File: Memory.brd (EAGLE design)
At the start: 106.7 x 54.3 mm, 14 parts, among them IC1 AT28C256ZIF, IC2 HM62256DIP, IC3 74LS139N, IC4 HM62256DIP

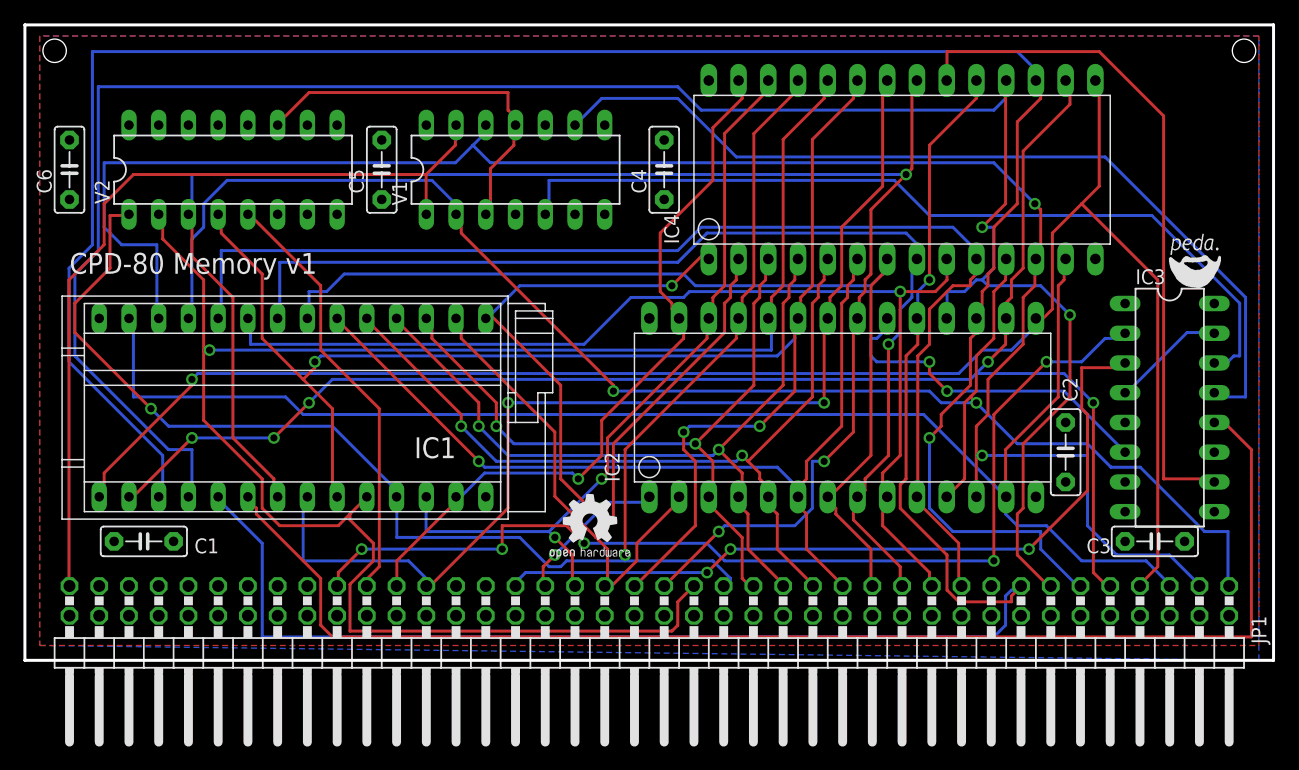
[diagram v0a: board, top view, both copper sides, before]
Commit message: Update Memory
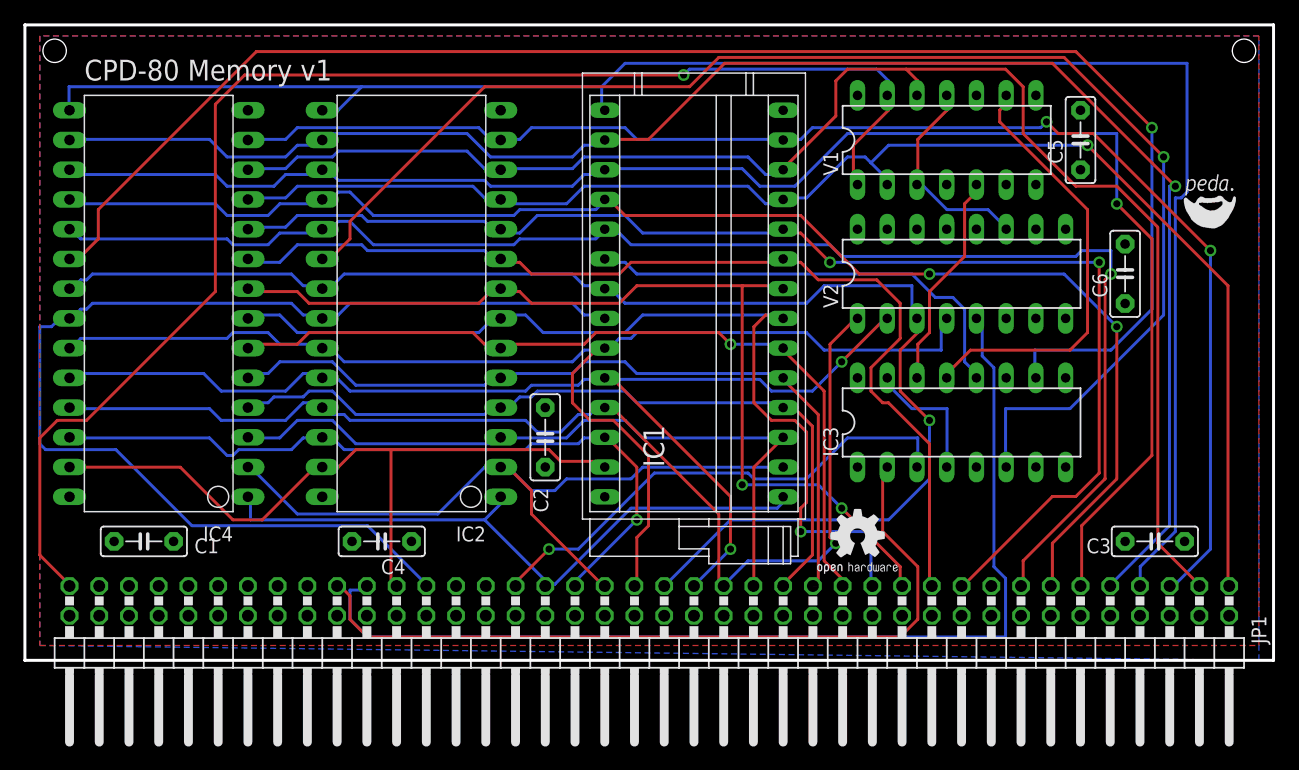
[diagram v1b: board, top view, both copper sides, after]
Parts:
- moved C6 90.6 mm to (92.7, 33.0)
- moved V2 62.9 mm to (78.7, 33.0)
- moved C5 59.7 mm to (88.9, 44.5)
- moved IC4 52.7 mm to (15.2, 22.9), turned to 90 degrees
- moved C2 44.5 mm to (43.2, 19.1), turned to 270 degrees
- moved C4 39.9 mm to (29.2, 10.2), turned to 180 degrees
- moved V1 36.9 mm to (77.5, 44.5)
- moved IC1 35.4 mm to (55.9, 30.5), turned to 90 degrees
- moved IC2 25.0 mm to (36.8, 22.9), turned to 90 degrees
- moved U$1 22.9 mm to (66.0, 6.35)
- moved IC3 17.8 mm to (78.7, 20.3), turned to 0 degrees
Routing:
- net N$1: track 29.9 -> 118.9 mm, vias 2 -> 1
- net N$9: track 58.7 -> 133.5 mm, vias 0 -> 1
- net N$2: track 113.6 -> 38.8 mm
- net D6: track 181.8 -> 121.4 mm
- net A9: track 157.2 -> 99.6 mm, vias 1 -> 2
- net N$3: track 73.3 -> 19.2 mm
- net !IOREQ: track 36.9 -> 89.0 mm
- net N$6: track 71.1 -> 119.3 mm, vias 0 -> 1
- net D5: track 182.4 -> 136.9 mm
- net N$5: track 76.7 -> 37.9 mm
- net A8: track 129.0 -> 100.2 mm, vias 2 -> 1
- net A10: track 148.5 -> 120.0 mm, vias 3 -> 1
- net D1: track 156.5 -> 128.5 mm, vias 2 -> 0
- net A15: track 67.2 -> 42.8 mm, vias 3 -> 1
- net A11: track 129.8 -> 107.2 mm, vias 3 -> 0
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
